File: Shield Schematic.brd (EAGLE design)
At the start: 53.3 x 94 mm, 31 parts, among them IC1 LM386N-1, IC2 LM1085IT-5.0, J2 POWER_JACK, U1 03540001ZXGY

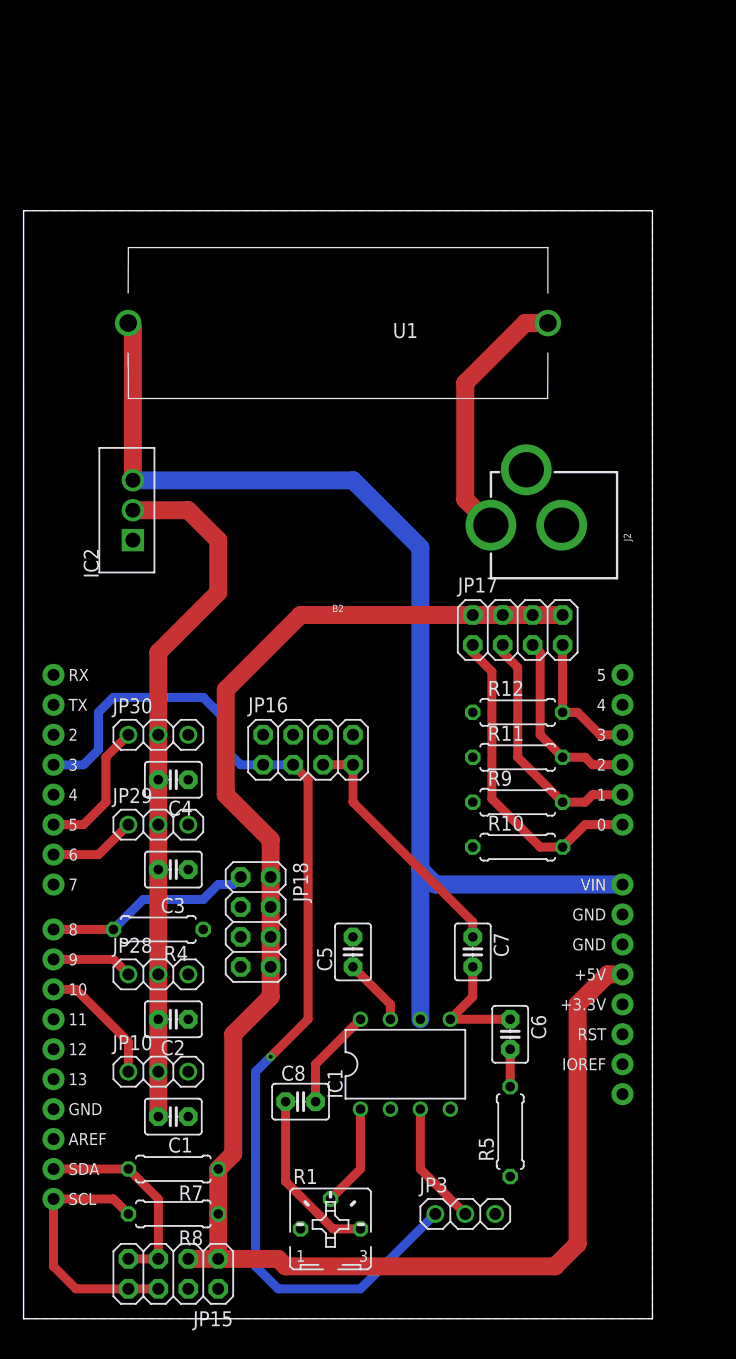
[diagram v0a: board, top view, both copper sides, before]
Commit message: Add files via upload
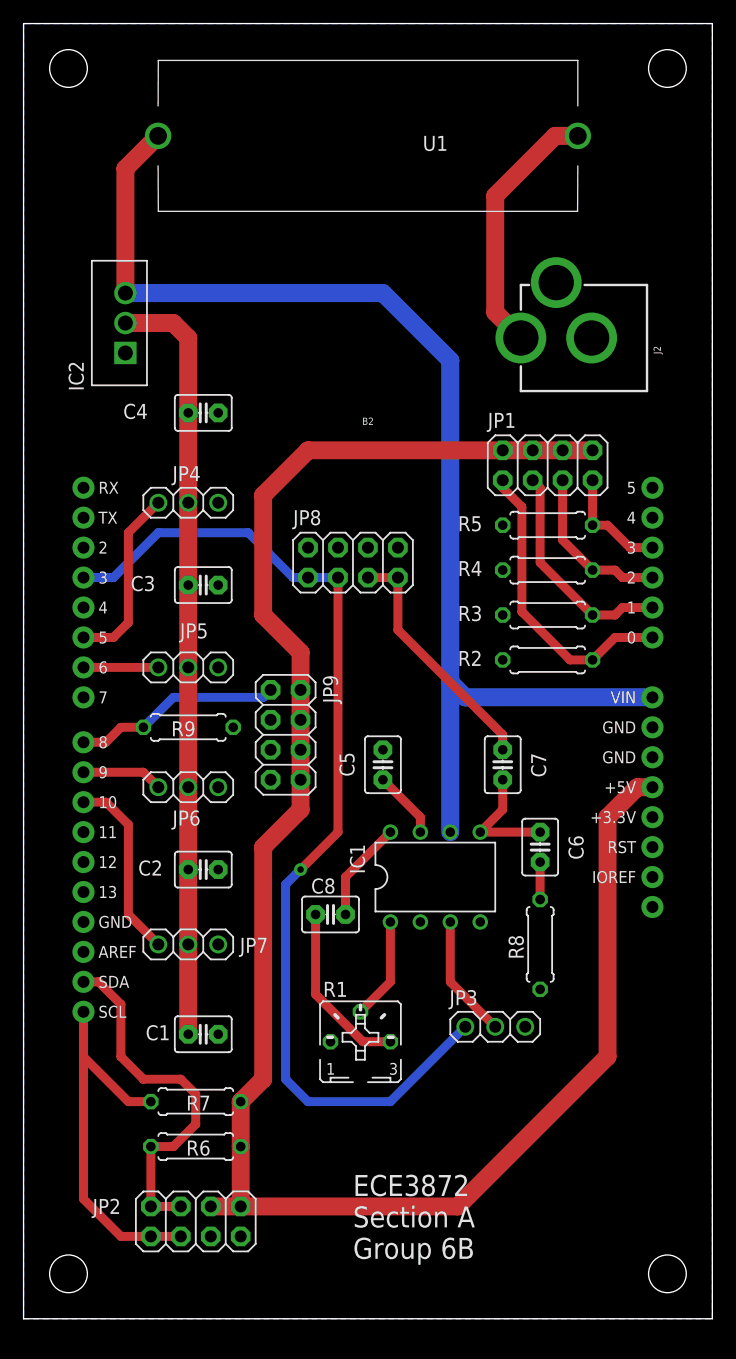
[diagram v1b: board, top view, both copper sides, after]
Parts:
- removed JP10, JP28, JP29, JP30: (no value), adafruit:1X03
- removed JP15, JP16, JP17, JP18: (no value), adafruit:2X04
- removed R10, R11, R12: (no value), resistor:0207/7
- added JP1, JP2, JP8, JP9: (no value), adafruit:2X04
- added JP4, JP5, JP6, JP7: (no value), adafruit:1X03
- added R2, R3, R6: (no value), resistor:0207/7
- moved R5 51.5 mm to (44.5, 67.3), turned to 0 degrees
- moved R4 44.9 mm to (44.5, 63.5), turned to 0 degrees
- moved R8 38.6 mm to (43.8, 31.8), turned to 90 degrees
- moved C4 31.2 mm to (15.2, 76.8)
- moved R9 28.7 mm to (14.0, 50.2), turned to 180 degrees
- moved C3 24.3 mm to (15.2, 62.2)
- moved C5 16.1 mm to (30.5, 47.0)
- moved C6 16.1 mm to (43.8, 40.0)
- moved C7 16.1 mm to (40.6, 47.0)
- moved IC1 16.1 mm to (34.9, 37.5)
- moved B2 16.1 mm to (29.2, 45.1)
- moved C8 16.1 mm to (26.0, 34.3)
- moved J2 16.1 mm to (55.9, 83.2)
- moved JP3 16.1 mm to (40.0, 24.8)
- moved R1 16.1 mm to (28.6, 23.5)
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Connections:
- net +5V_SERVO: now also JP4.2, JP5.2, JP6.2, JP7.2; no longer JP10.2, JP28.2, JP29.2, JP30.2
- net +5V_UNO: now also JP1.2, JP1.4, JP1.6, JP1.8, JP2.1, JP2.3, JP9.2, JP9.4, JP9.6, JP9.8, R6.1; no longer JP15.1, JP15.3, JP17.2, JP17.4, JP17.6, JP17.8, JP18.2, JP18.4, JP18.6, JP18.8, R8.1
- net ACTION_BUTTON: now also JP1.7, R5.2; no longer JP17.7, R12.2
- net GND: now also JP2.2, JP2.4, JP4.3, JP5.3, JP6.3, JP7.3, JP8.2, JP8.4, JP8.6, JP8.8, R2.1, R3.1, R8.1; no longer JP10.3, JP15.2, JP15.4, JP16.2, JP16.4, JP16.6, JP16.8, JP28.3, JP29.3, JP30.3, R10.1, R11.1, R12.1
- net N$8: now also R8.2; no longer R5.2
- net PLAYLIVE_SWITCH: now also JP1.3, R3.2; no longer JP17.3, R9.2
- net PLAYRECORDING_SWITCH: now also JP1.5, R4.2; no longer JP17.5, R11.2
- net RECORD_SWITCH: now also JP1.1, R2.2; no longer JP17.1, R10.2
- net RESET_BUTTON: now also JP9.1, R9.2; no longer JP18.1, R4.2
- net SCL: now also JP2.6, JP2.8, R7.2; no longer JP15.6, JP15.8, R8.2
- net SDA: now also JP2.5, JP2.7, R6.2; no longer JP15.5, JP15.7, R7.2
- net SERVO1: now also JP4.1; no longer JP30.1
- net SERVO2: now also JP5.1; no longer JP29.1
- net SERVO3: now also JP6.1; no longer JP28.1
- net SERVO4: now also JP7.1; no longer JP10.1
- net SPEAKER: now also JP8.5, JP8.7; no longer JP16.5, JP16.7
- net TONE_IN: now also JP8.1, JP8.3; no longer JP16.1, JP16.3
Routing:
- net +5V_UNO: track 142.1 -> 157.4 mm
- net SDA: track 17.6 -> 30.8 mm
- net SCL: track 22.3 -> 32.7 mm
- net +5V_SERVO: track 59.3 -> 64.9 mm
- net SERVO4: track 10.7 -> 15.8 mm
- net TONE_IN: track 92.0 -> 87.8 mm
- net +12V: track 97.9 -> 102.1 mm
- net SERVO1: track 11.7 -> 15.5 mm
- net RECORD_SWITCH: track 27.3 -> 25.4 mm
- net PLAYRECORDING_SWITCH: track 15.9 -> 14.0 mm
- net PLAYLIVE_SWITCH: track 20.8 -> 18.9 mm
- net ACTION_BUTTON: track 11.6 -> 9.68 mm
- net SERVO2: track 7.40 -> 6.35 mm
- net SPEAKER: track 21.4 -> 20.8 mm
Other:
- board size 53.3 x 94 mm -> 58.4 x 109.9 mm
- board text added: "ECE3872 Section A Group 6B"
